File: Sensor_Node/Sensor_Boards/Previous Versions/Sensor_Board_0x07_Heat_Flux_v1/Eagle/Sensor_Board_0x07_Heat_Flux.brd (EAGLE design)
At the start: 31.5 x 57 mm, 24 parts, among them IC1 MCP3911A0-E/SS, IC2 4066D, U1 PIC16F1825-I/ST-TSSOP14, X1 22-23-2041

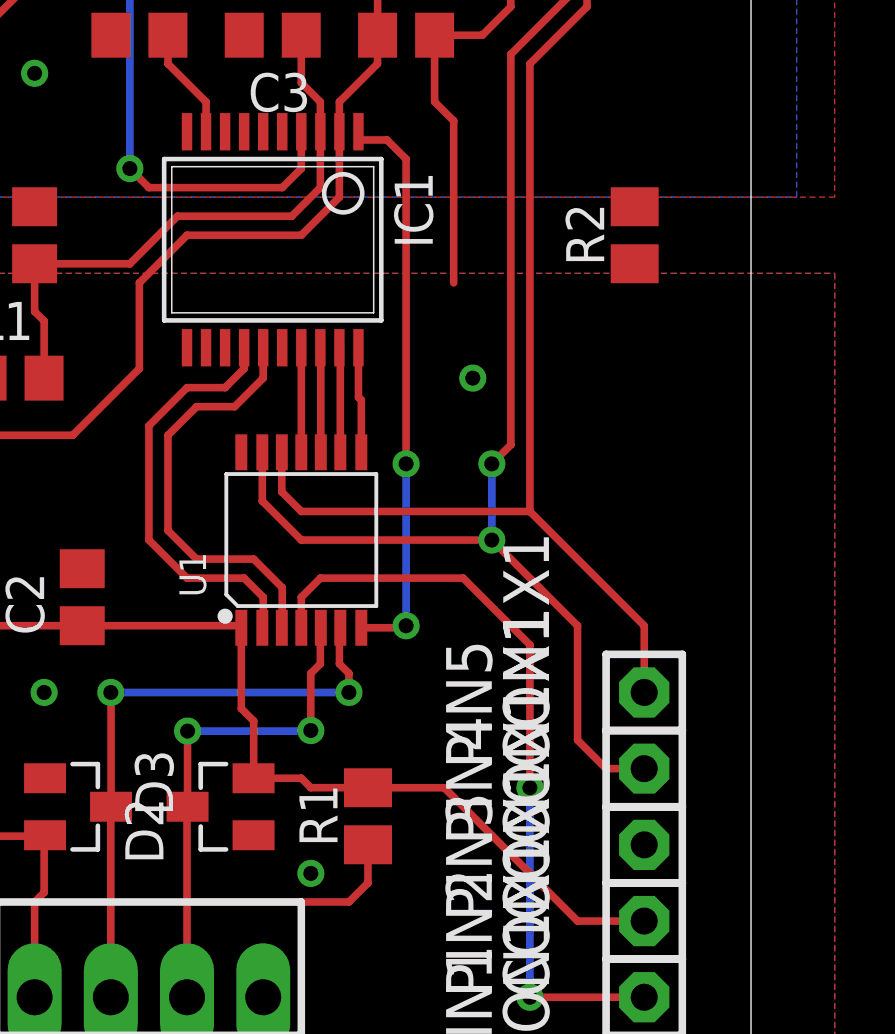
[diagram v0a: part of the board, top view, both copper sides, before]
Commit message: Work on heat flux sensor continued
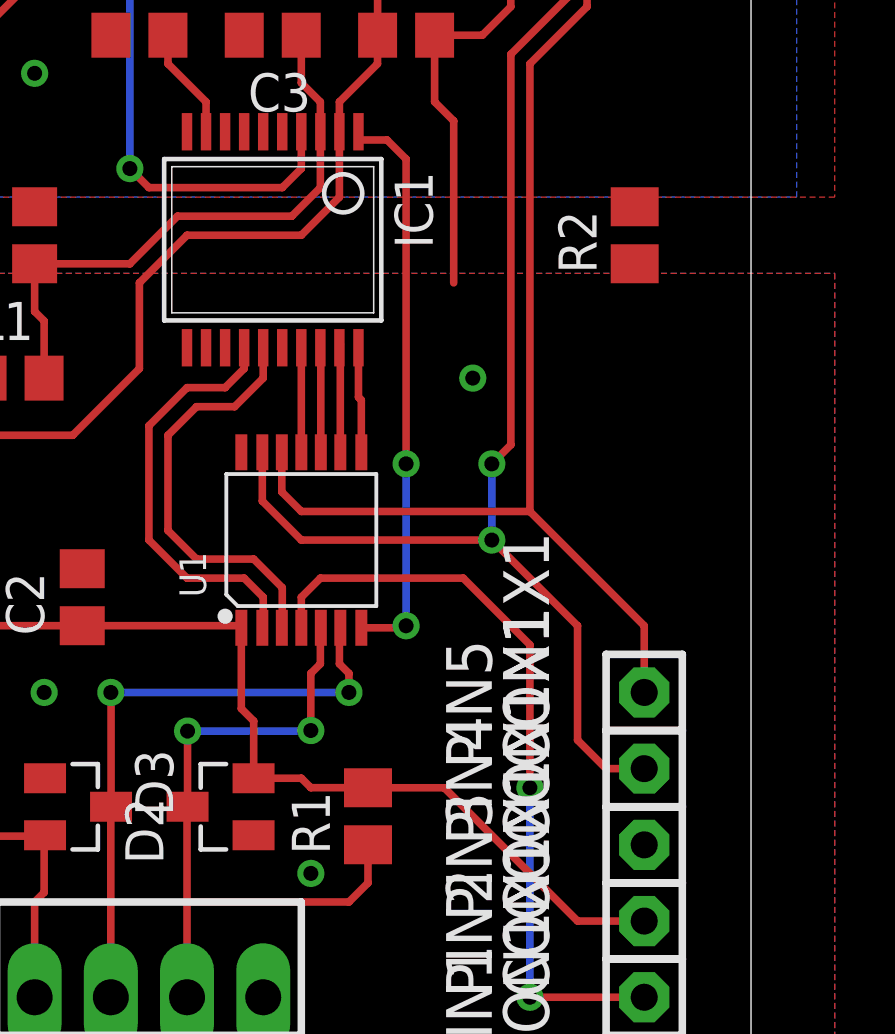
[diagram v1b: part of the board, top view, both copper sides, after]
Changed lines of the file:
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@@
 <?xml version="1.0" encoding="utf-8"?>
 <!DOCTYPE eagle SYSTEM "eagle.dtd">
-<eagle version="7.5.0">
+<eagle version="9.0.1">
 <drawing>
 <settings>
 <setting alwaysvectorfont="no"/>
+<setting keepoldvectorfont="yes"/>
 <setting verticaltext="up"/>
 </settings>
@@
 <param name="dpMaxLengthDifference" value="10mm"/>
 <param name="dpGapFactor" value="2.5"/>
-<param name="checkGrid" value="0"/>
 <param name="checkAngle" value="0"/>
 <param name="checkFont" value="1"/>
 <param name="checkRestrict" value="1"/>
+<param name="checkStop" value="0"/>
+<param name="checkValues" value="0"/>
 <param name="useDiameter" value="13"/>
 <param name="maxErrors" value="50"/>
@@
 <element name="D2" library="LEDXLamp" package="SOT23" value="BAV99" x="13.8176" y="10.16" rot="R90"/>
 <element name="D3" library="LEDXLamp" package="SOT23" value="BAV99" x="9.0678" y="10.16" rot="R270"/>
-<element name="IC1" library="heatflow" package="SSOP20" value="MCP3911A0-E/SS" x="15.5575" y="29.21" rot="R180"/>
-<element name="IC2" library="40xx" package="SO14" value="4066D" x="15.24" y="42.2275" rot="R180"/>
+<element name="IC1" library="heatflow" package="SSOP20" value="MCP3911A0-E/SS" x="15.5575" y="29.21" rot="R180">
+<attribute name="SPICEPREFIX" value="X" x="15.5575" y="29.21" size="1.778" layer="27" rot="R180" display="off"/>
+</element>
+<element name="IC2" library="40xx" library_urn="urn:adsk.eagle:library:80" package="SO14" package3d_urn="urn:adsk.eagle:package:823/2" value="4066D" x="15.24" y="42.2275" rot="R180"/>
 <element name="J1" library="Stecker_Pins" package="CON2X1" value="" x="16.51" y="53.6575" rot="R90"/>
 <element name="L1" library="heatflow2" package="0805" value="74279220601" x="6.985" y="24.4475"/>
@@
 <element name="PIN4" library="Stecker_Pins" package="CON1X1" value="CON1X1" x="27.94" y="8.89" rot="R90"/>
 <element name="PIN5" library="Stecker_Pins" package="CON1X1" value="CON1X1" x="27.94" y="11.43" rot="R90"/>
-<element name="R1" library="resistor" package="M0805" value="10k" x="18.7325" y="9.8425" rot="R90"/>
-<element name="R2" library="resistor" package="M0805" value="0" x="27.6225" y="29.21" rot="R90"/>
+<element name="R1" library="resistor" library_urn="urn:adsk.eagle:library:348" package="M0805" package3d_urn="urn:adsk.eagle:package:26079/1" value="10k" x="18.7325" y="9.8425" rot="R90"/>
+<element name="R2" library="resistor" library_urn="urn:adsk.eagle:library:348" package="M0805" package3d_urn="urn:adsk.eagle:package:26079/1" value="0" x="27.6225" y="29.21" rot="R90"/>
 <element name="U1" library="heatflow" package="TSSOP14-0.65-5X4.4MM" value="PIC16F1825-I/ST-TSSOP14" x="16.51" y="19.05">
 <attribute name="MPN" value="PIC16F1825-I/ST" x="16.51" y="19.05" size="1.778" layer="27" display="off"/>
 </element>
 <element name="X1" library="heatflow" package="22-23-2041" value="22-23-2041" x="11.43" y="3.81" rot="R180">
+<attribute name="MF" value="MOLEX" x="11.43" y="3.81" size="1.778" layer="27" rot="R180" display="off"/>
+<attribute name="MPN" value="22-23-2041" x="11.43" y="3.81" size="1.778" layer="27" rot="R180" display="off"/>
+<attribute name="OC_FARNELL" value="1462920" x="11.43" y="3.81" size="1.778" layer="27" rot="R180" display="off"/>
 <attribute name="OC_NEWARK" value="38C0355" x="11.43" y="3.81" size="1.778" layer="27" rot="R180" display="off"/>
-<attribute name="OC_FARNELL" value="1462920" x="11.43" y="3.81" size="1.778" layer="27" rot="R180" display="off"/>
-<attribute name="MPN" value="22-23-2041" x="11.43" y="3.81" size="1.778" layer="27" rot="R180" display="off"/>
-<attribute name="MF" value="MOLEX" x="11.43" y="3.81" size="1.778" layer="27" rot="R180" display="off"/>
 </element>
 <element name="C10" library="heatflow" package="C0805" value="1u" x="4.1275" y="10.16" rot="R90"/>
@@
 </board>
 </drawing>
+<compatibility>
+<note version="8.2" severity="warning">
+Since Version 8.2, EAGLE supports online libraries. The ids
+of those online libraries will not be understood (or retained)
+with this version.
+</note>
+<note version="8.3" severity="warning">
+Since Version 8.3, EAGLE supports URNs for individual library
+assets (packages, symbols, and devices). The URNs of those assets
+will not be understood (or retained) with this version.
+</note>
+<note version="8.3" severity="warning">
+Since Version 8.3, EAGLE supports the association of 3D packages
+with devices in libraries, schematics, and board files. Those 3D
+packages will not be understood (or retained) with this version.
+</note>
+</compatibility>
 </eagle>
